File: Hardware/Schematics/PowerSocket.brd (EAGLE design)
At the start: 100 x 50 mm, 74 parts, among them T1 BT138-V, T2 BT138-V, T3 BT138-V, T4 BT138-V, T5 BT138-V, T6 BT138-V

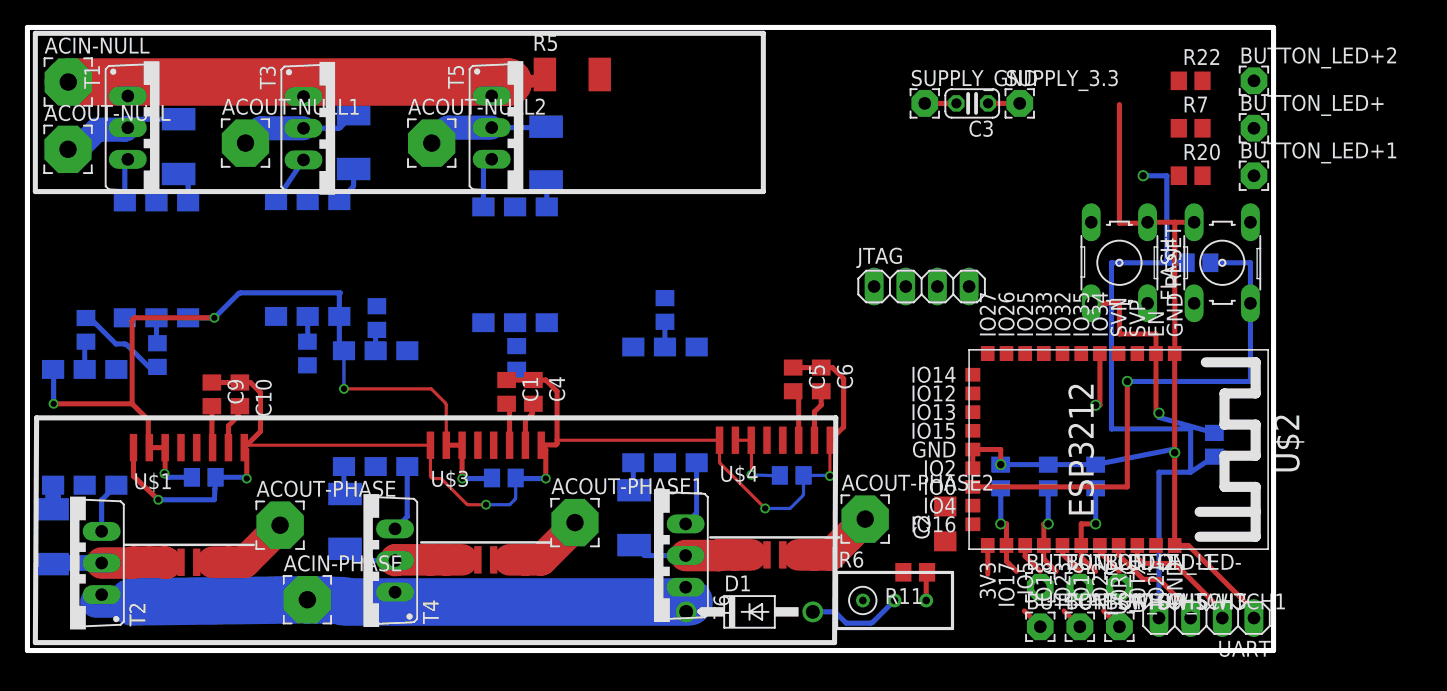
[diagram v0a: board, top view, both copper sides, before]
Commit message: Routed board.
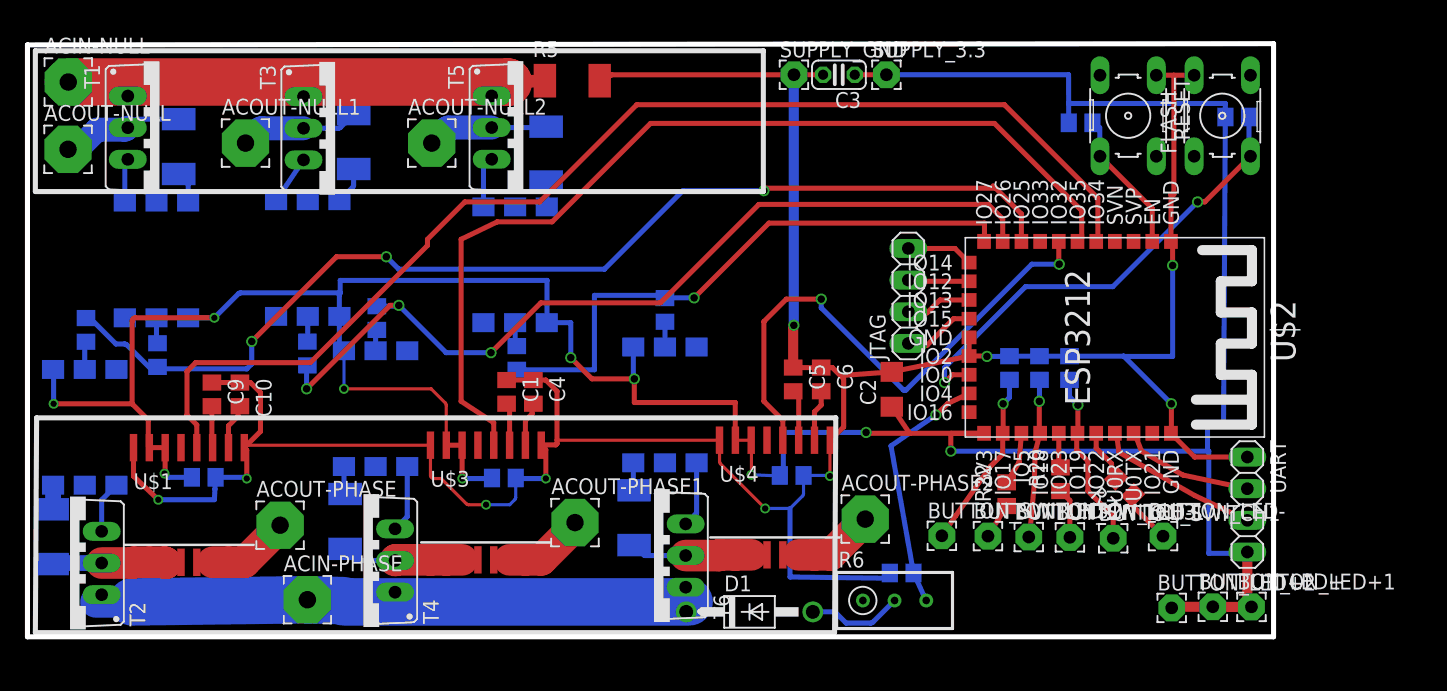
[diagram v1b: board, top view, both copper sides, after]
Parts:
- moved BUTTON_LED+2 42.8 mm to (91.8, 3.42)
- moved BUTTON_LED+ 38.5 mm to (95.1, 3.51)
- moved R22 36.3 mm to (78.6, 12.5), turned to 90 degrees
- moved BUTTON_LED+1 34.6 mm to (98.2, 3.50)
- moved R7 29.3 mm to (88.0, 13.1), turned to 135 degrees
- moved R1 28.0 mm to (84.5, 42.4), turned to 0 degrees
- moved R20 26.5 mm to (82.9, 13.7), turned to 90 degrees
- moved R2 12.1 mm to (97.1, 42.8)
- moved RESET 11.8 mm to (88.3, 42.9)
- moved FLASH 11.8 mm to (95.9, 42.9)
- moved C2 11.6 mm to (69.4, 21.0)
- moved C3 10.9 mm to (65.1, 46.2)
- moved SUPPLY_3.3 10.9 mm to (68.9, 46.2)
- moved BUTTON_SWITCH5 10.8 mm to (73.4, 9.21)
- moved SUPPLY_GND 10.7 mm to (61.5, 46.2)
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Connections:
- net N$3: now also U$2.IO4; no longer U$2.IO33
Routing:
- net VCC: track 140.7 -> 259.1 mm, vias 7 -> 10
- net N$12: track 4.49 -> 95.3 mm, vias 1 -> 0
- net N$8: track 7.15 -> 88.5 mm, vias 0 -> 3
- net N$11: track 0.00 -> 76.8 mm
- net N$25: track 0.00 -> 71.1 mm, vias 0 -> 3
- net GND: track 180.6 -> 232.6 mm, vias 8 -> 10
- net N$54: track 0.00 -> 47.7 mm, vias 0 -> 1
- net N$41: track 0.00 -> 44.1 mm, vias 0 -> 2
- net N$3: track 2.27 -> 20.4 mm, vias 0 -> 1
- net N$2: track 19.2 -> 11.6 mm, vias 1 -> 0
- net N$59: track 0.00 -> 5.82 mm
- net N$56: track 0.00 -> 5.35 mm
- net N$58: track 0.00 -> 5.34 mm
- net N$7: track 43.5 -> 38.3 mm, vias 1 -> 2
- net N$39: track 9.26 -> 14.4 mm
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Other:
- board size 100 x 50 mm -> 100 x 47.6 mm
